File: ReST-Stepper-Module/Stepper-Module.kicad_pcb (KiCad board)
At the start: 2 copper layers, 46 x 32.8 mm, 32 parts

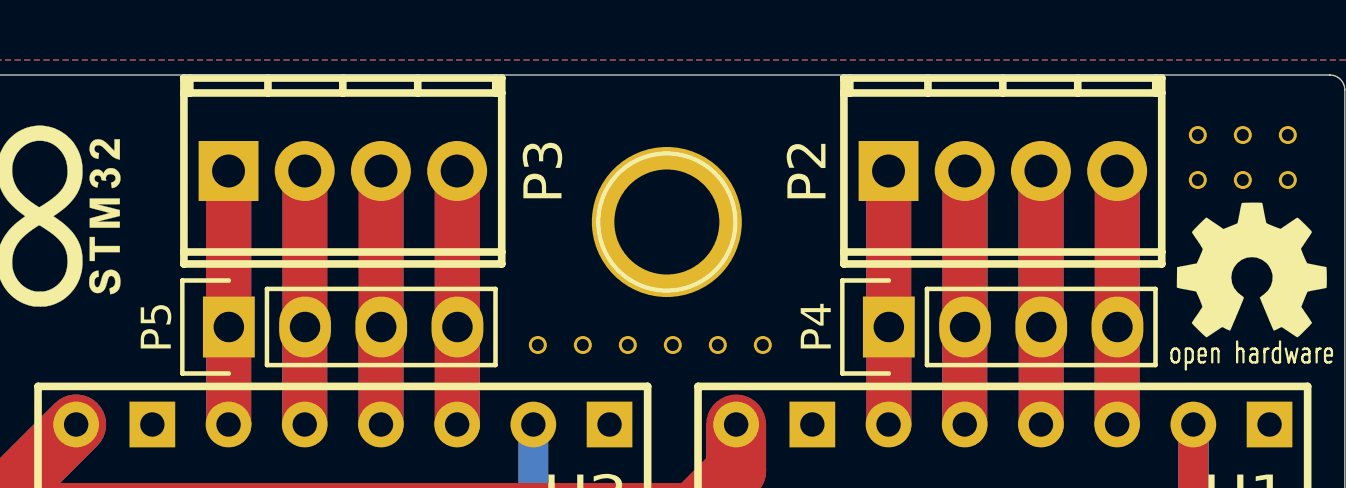
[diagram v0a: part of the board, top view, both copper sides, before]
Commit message: Final release
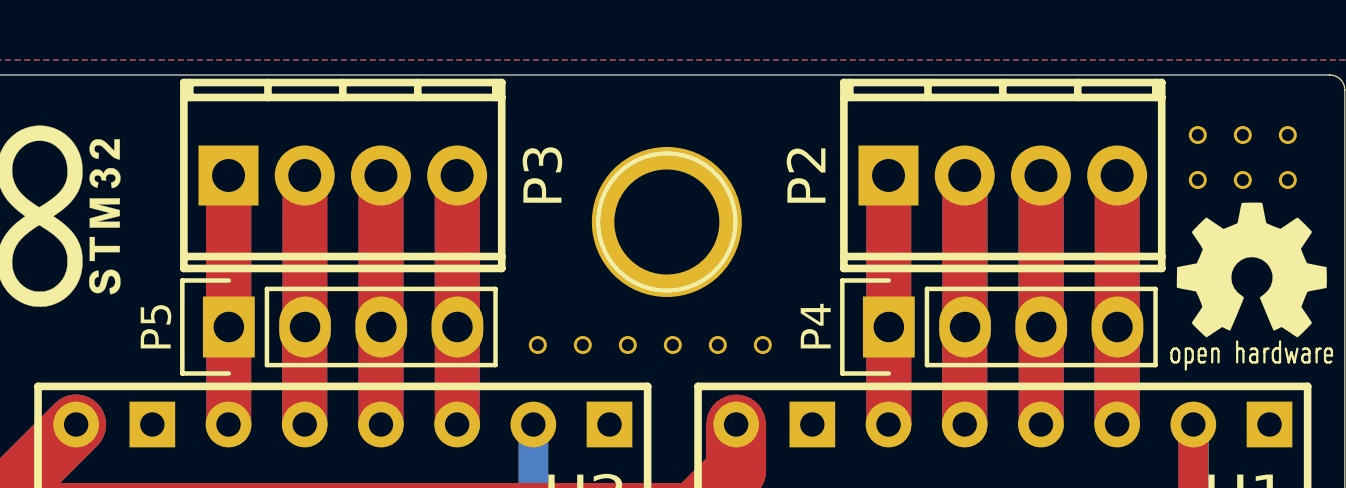
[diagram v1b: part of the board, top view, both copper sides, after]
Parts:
- moved P2 0.15 mm to (137.0, 81.3)
- moved P3 0.15 mm to (115.0, 81.3)
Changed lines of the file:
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@@
     (links 79)
     (no_connects 0)
-    (area 102.394999 77.994999 148.405001 110.805001)
+    (area 100.8832 75.12512 149.000001 111.500001)
     (thickness 1.6)
     (drawings 9)
@@
     (visible_elements 7FFFFFFF)
     (pcbplotparams
-      (layerselection 0x00030_80000001)
-      (usegerberextensions false)
+      (layerselection 0x010f0_80000001)
+      (usegerberextensions true)
       (excludeedgelayer true)
       (linewidth 0.100000)
@@
       (outputformat 1)
       (mirror false)
-      (drillshape 1)
+      (drillshape 0)
       (scaleselection 1)
-      (outputdirectory ""))
+      (outputdirectory ../Gerber/Stepper/))
   )
   (net 0 "")
@@
   )
   (module 2:mpt_0,5%2f4-2,54 (layer F.Cu)
-    (at 137 81.2 180)
+    (at 137 81.35 180)
     (descr "4-way 2.54mm pitch terminal block, Phoenix MPT series")
     (fp_text reference P2 (at 6.5 0 270) (layer F.SilkS)
@@
   )
   (module 2:mpt_0,5%2f4-2,54 (layer F.Cu)
-    (at 115 81.2 180)
+    (at 115 81.35 180)
     (descr "4-way 2.54mm pitch terminal block, Phoenix MPT series")
     (fp_text reference P3 (at -6.7 0 270) (layer F.SilkS)
